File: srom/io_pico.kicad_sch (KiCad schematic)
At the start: 2 parts, among them J201 Conn_01x03_Female, U201 Pico-2 IO

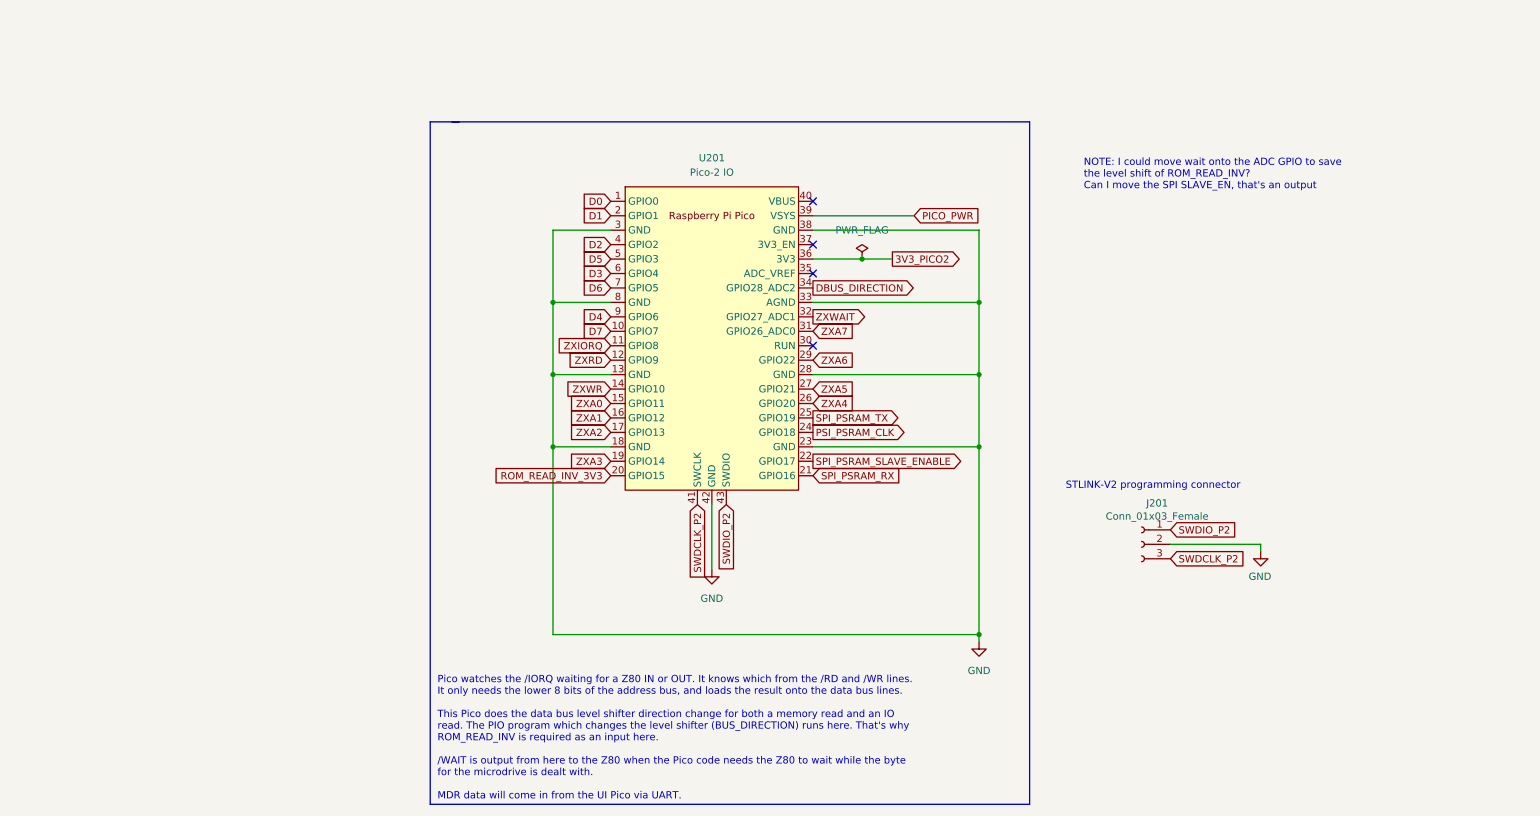
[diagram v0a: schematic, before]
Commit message: start updating schematic for next board
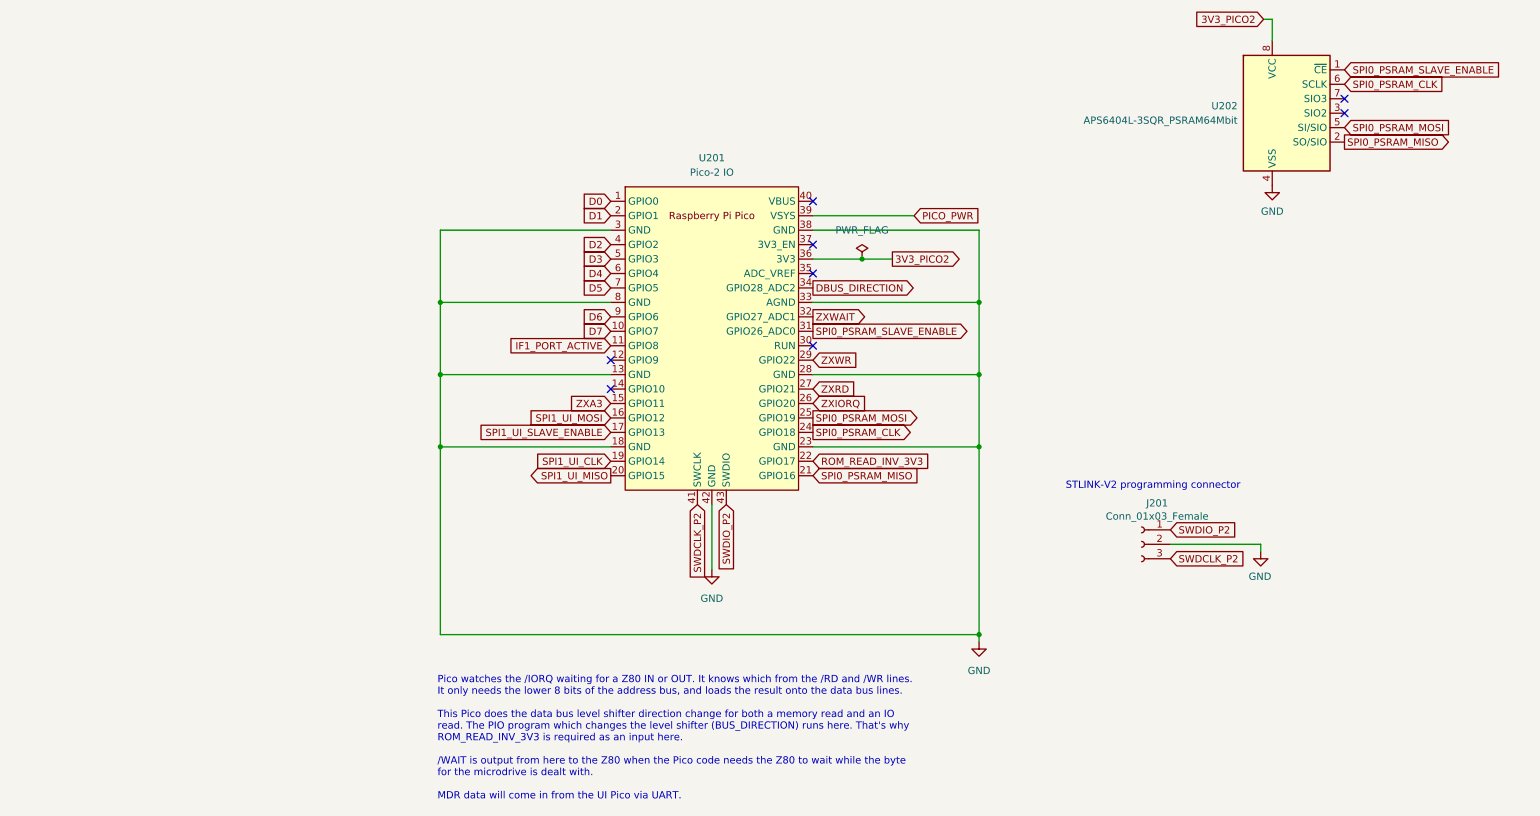
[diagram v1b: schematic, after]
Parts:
- added U202: APS6404L-3SQR_PSRAM64Mbit, Package_SO:SOIC-8_3.9x4.9mm_P1.27mm, symbol Memory_RAM:APS6404L-3SQR_PSRAM64Mbit
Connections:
- net SPI_PSRAM_SLAVE_ENABLE is gone; now on net ROM_READ_INV_3V3: U201.22 (GPIO17)
- net ZXA0 is gone; now on net ZXA3: U201.15 (GPIO11)
- net ZXA4 is gone; now on net ZXIORQ: U201.26 (GPIO20)
- net ZXA5 is gone; now on net ZXRD: U201.27 (GPIO21)
- net ZXA6 is gone; now on net ZXWR: U201.29 (GPIO22)
- net 3V3_PICO2: now also U202.8 (VCC)
- net D3: now also U201.5 (GPIO3); no longer U201.6 (GPIO4)
- net D4: now also U201.6 (GPIO4); no longer U201.9 (GPIO6)
- net D5: now also U201.7 (GPIO5); no longer U201.5 (GPIO3)
- net D6: now also U201.9 (GPIO6); no longer U201.7 (GPIO5)
- net GND: now also U202.4 (VSS)
- net ROM_READ_INV_3V3: no longer U201.20 (GPIO15)
- net ZXA3: no longer U201.19 (GPIO14)
- net ZXIORQ: no longer U201.11 (GPIO8)
- net ZXRD: no longer U201.12 (GPIO9)
- net ZXWR: no longer U201.14 (GPIO10)
- net PSI_PSRAM_CLK renamed SPI0_PSRAM_CLK
- net SPI0_PSRAM_CLK: now also U202.6 (SCLK)
- net SPI_PSRAM_RX renamed SPI0_PSRAM_MISO
- net SPI0_PSRAM_MISO: now also U202.2 (SO/SIO)
- net SPI_PSRAM_TX renamed SPI0_PSRAM_MOSI
- net SPI0_PSRAM_MOSI: now also U202.5 (SI/SIO)
- net ZXA1 renamed SPI1_UI_MOSI
- net ZXA2 renamed SPI1_UI_SLAVE_ENABLE
- net ZXA7 renamed SPI0_PSRAM_SLAVE_ENABLE
- net SPI0_PSRAM_SLAVE_ENABLE: now also U202.1 (~{CE})
- new net IF1_PORT_ACTIVE: U201.11 (GPIO8)
- new net SPI1_UI_CLK: U201.19 (GPIO14)
- new net SPI1_UI_MISO: U201.20 (GPIO15)
- no-connect marks 4 -> 8
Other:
- note added: "Pico watches the /IORQ waiting for a Z80 IN or OUT. It knows which from the /RD and /WR lines. It only needs the lower 8 bits of the address bus, and loads the result onto the data bus lines. This Pico does the data bus level shifter direction change for both a memory read and an IO read. The PIO program which changes the level shifter (BUS_DIRECTION) runs here. That's why ROM_READ_INV_3V3 is req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"
- note removed: "NOTE: I could move wait onto the ADC GPIO to save the level shift of ROM_READ_INV? Can I move the SPI SLAVE_EN, that's an output"
- note removed: "Pico watches the /IORQ waiting for a Z80 IN or OUT. It knows which from the /RD and /WR lines. It only needs the lower 8 bits of the address bus, and loads the result onto the data bus lines. This Pico does the data bus level shifter direction change for both a memory read and an IO read. The PIO program which changes the level shifter (BUS_DIRECTION) runs here. That's why ROM_READ_INV is require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"

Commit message: first draft of layout of board 2
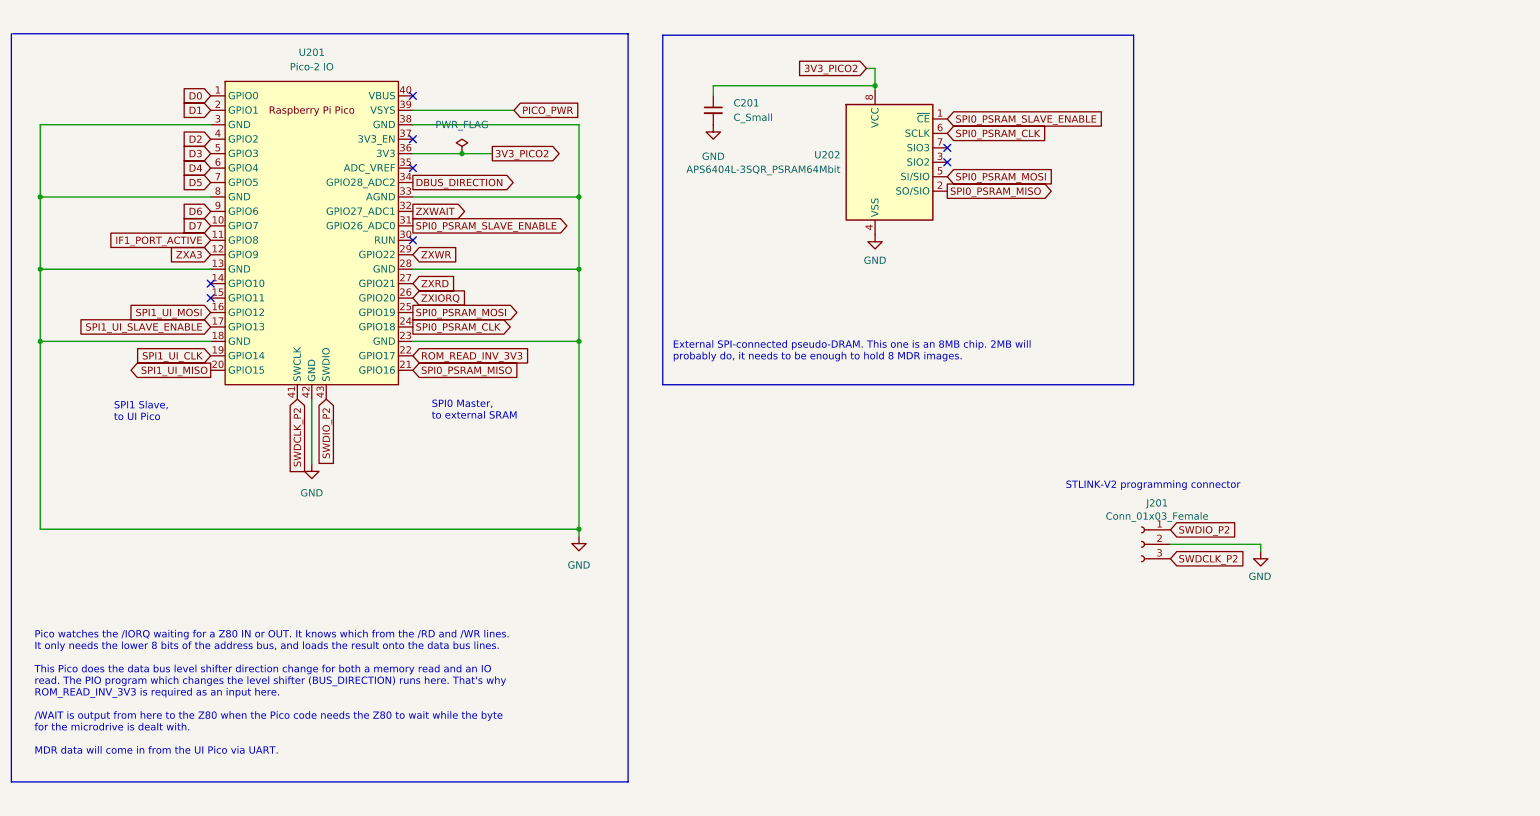
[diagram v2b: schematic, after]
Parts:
- added C201: C_Small, Capacitor_SMD:C_1206_3216Metric, symbol Device:C_Small
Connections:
- net 3V3_PICO2: now also C201.1
- net GND: now also C201.2
- net ZXA3: now also U201.12 (GPIO9); no longer U201.15 (GPIO11)
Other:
- note added: "External SPI-connected pseudo-DRAM. This one is an 8MB chip. 2MB will probably do, it needs to be enough to hold 8 MDR images."
- note added: "SPI0 Master, to external SRAM"
- note added: "SPI1 Slave, to UI Pico"
- moved on the sheet: U201, U202

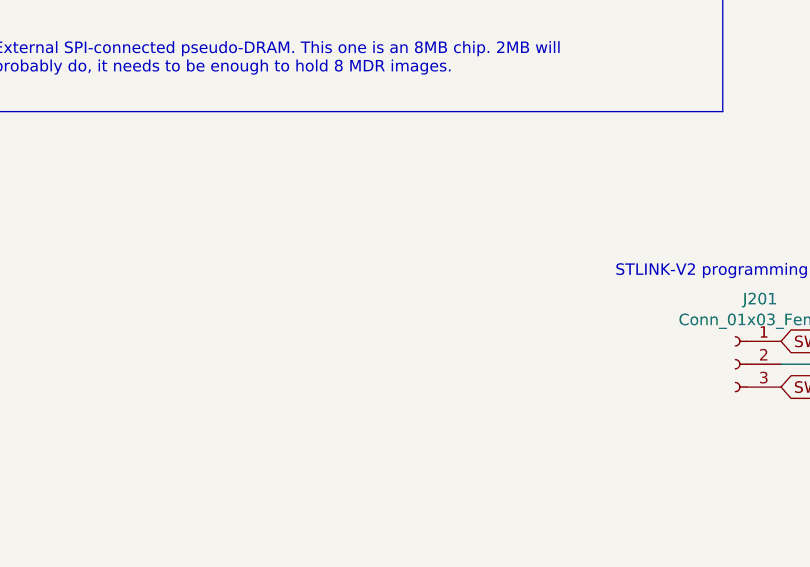
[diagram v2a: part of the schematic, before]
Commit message: more work on the layout of board 2
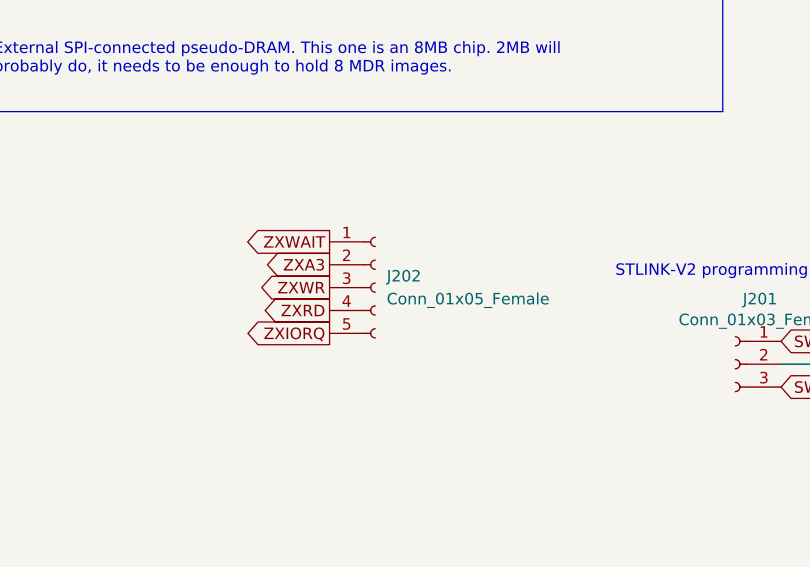
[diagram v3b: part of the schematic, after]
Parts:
- added J202: Conn_01x05_Female, Connector_PinHeader_2.54mm:PinHeader_1x05_P2.54mm_Vertical, symbol Connector:Conn_01x05_Female
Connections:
- net ZXA3: now also J202.2 (Pin_2)
- net ZXIORQ: now also J202.5 (Pin_5)
- net ZXRD: now also J202.4 (Pin_4)
- net ZXWAIT: now also J202.1 (Pin_1)
- net ZXWR: now also J202.3 (Pin_3)
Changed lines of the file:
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@@
     (effects (font (size 1.27 1.27)) (justify left bottom))
   )
+  (global_label "ZXIORQ" (shape output) (at 175.26 106.426 180) (fields_autoplaced)
+    (effects (font (size 1.27 1.27)) (justify right))
+    (property "Intersheet References" "${INTERSHEET_REFS}" (id 0) (at 165.8921 106.5054 0)
+      (effects (font (size 1.27 1.27)) (justify right) hide)
+    )
+  )
+  (global_label "ZXWR" (shape output) (at 175.26 101.346 180) (fields_autoplaced)
+    (effects (font (size 1.27 1.27)) (justify right))
+    (property "Intersheet References" "${INTERSHEET_REFS}" (id 0) (at 167.7064 101.4254 0)
+      (effects (font (size 1.27 1.27)) (justify right) hide)
+    )
+  )
+  (global_label "ZXA3" (shape output) (at 175.26 98.806 180) (fields_autoplaced)
+    (effects (font (size 1.27 1.27)) (justify right))
+    (property "Intersheet References" "${INTERSHEET_REFS}" (id 0) (at 168.1298 98.7266 0)
+      (effects (font (size 1.27 1.27)) (justify right) hide)
+    )
+  )
   (global_label "SPI1_UI_MISO" (shape output) (at 56.642 79.248 180) (fields_autoplaced)
     (effects (font (size 1.27 1.27)) (justify right))
@@
     )
   )
+  (global_label "ZXRD" (shape output) (at 175.26 103.886 180) (fields_autoplaced)
+    (effects (font (size 1.27 1.27)) (justify right))
+    (property "Intersheet References" "${INTERSHEET_REFS}" (id 0) (at 167.8879 103.9654 0)
+      (effects (font (size 1.27 1.27)) (justify right) hide)
+    )
+  )
   (global_label "ZXWAIT" (shape output) (at 92.202 51.308 0) (fields_autoplaced)
     (effects (font (size 1.27 1.27)) (justify left))
@@
     (effects (font (size 1.27 1.27)) (justify right))
     (property "Intersheet References" "${INTERSHEET_REFS}" (id 0) (at 38.3841 56.3086 0)
+      (effects (font (size 1.27 1.27)) (justify right) hide)
+    )
+  )
+  (global_label "ZXWAIT" (shape output) (at 175.26 96.266 180) (fields_autoplaced)
+    (effects (font (size 1.27 1.27)) (justify right))
+    (property "Intersheet References" "${INTERSHEET_REFS}" (id 0) (at 166.3155 96.1866 0)
       (effects (font (size 1.27 1.27)) (justify right) hide)
     )
@@
     (pin "2")
   )
+  (symbol (lib_id "Connector:Conn_01x05_Female") (at 180.34 101.346 0) (unit 1)
+    (in_bom yes) (on_board yes) (fields_autoplaced)
+    (property "Reference" "J202" (id 0) (at 181.61 100.0759 0)
+      (effects (font (size 1.27 1.27)) (justify left))
+    )
+    (property "Value" "Conn_01x05_Female" (id 1) (at 181.61 102.6159 0)
+      (effects (font (size 1.27 1.27)) (justify left))
+    )
+    (property "Footprint" "Connector_PinHeader_2.54mm:PinHeader_1x05_P2.54mm_Vertical" (id 2) (at 180.34 101.346 0)
+      (effects (font (size 1.27 1.27)) hide)
+    )
+    (property "Datasheet" "~" (id 3) (at 180.34 101.346 0)
+      (effects (font (size 1.27 1.27)) hide)
+    )
+    (pin "1")
+    (pin "2")
+    (pin "3")
+    (pin "4")
+    (pin "5")
+  )
   (symbol (lib_id "pico-sym:Pico") (at 74.422 55.118 0) (unit 1)
